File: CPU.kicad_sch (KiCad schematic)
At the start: 56 parts, among them Y1 X322524MKB4SI

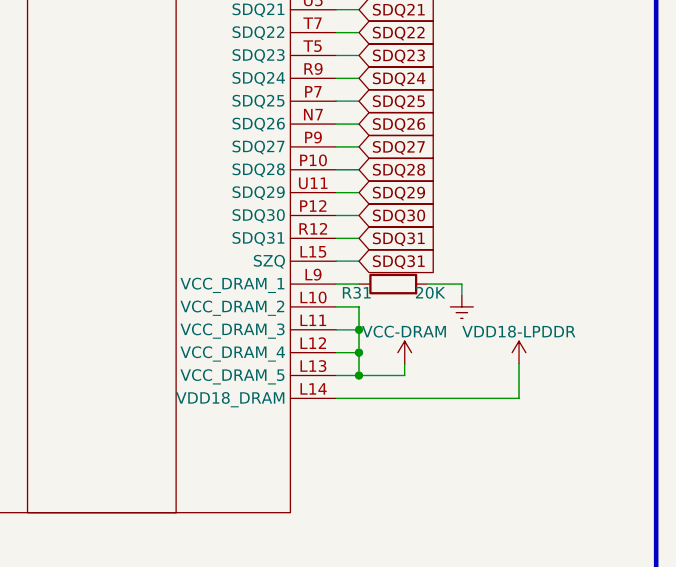
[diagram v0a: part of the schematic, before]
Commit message: Пытаюсь сделать трассировку DDК
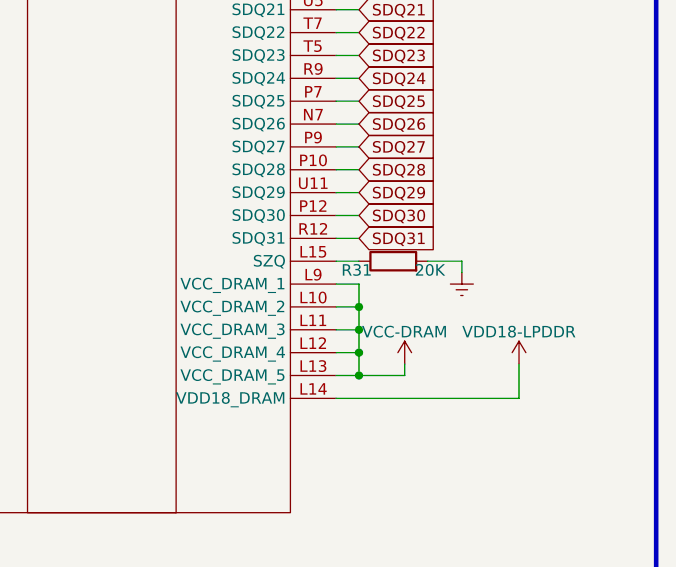
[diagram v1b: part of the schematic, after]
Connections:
- net SDQ31: no longer DD1.L15 (SZQ)
- net VCC-DRAM: now also DD1.L9 (VCC_DRAM_1)
- net at R31.1: now also DD1.L15 (SZQ); no longer DD1.L9 (VCC_DRAM_1)
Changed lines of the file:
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@@
 	)
 	(junction
+		(at 369.57 149.86)
+		(diameter 0)
+		(color 0 0 0 0)
+	)
+	(junction
 		(at 260.35 228.6)
 		(diameter 0)
@@
 	(wire
 		(pts
+			(xy 369.57 147.32) (xy 369.57 149.86)
+		)
+		(stroke
+			(width 0)
+			(type default)
+		)
+	)
+	(wire
+		(pts
 			(xy 254 228.6) (xy 260.35 228.6)
 		)
@@
 	(wire
 		(pts
+			(xy 367.03 147.32) (xy 369.57 147.32)
+		)
+		(stroke
+			(width 0)
+			(type default)
+		)
+	)
+	(wire
+		(pts
 			(xy 128.27 68.58) (xy 125.73 68.58)
 		)
@@
 	(wire
 		(pts
+			(xy 381 146.05) (xy 381 144.78)
+		)
+		(stroke
+			(width 0)
+			(type default)
+		)
+	)
+	(wire
+		(pts
 			(xy 128.27 83.82) (xy 125.73 83.82)
 		)
@@
 	(wire
 		(pts
-			(xy 381 148.59) (xy 381 147.32)
-		)
-		(stroke
-			(width 0)
-			(type default)
-		)
-	)
-	(wire
-		(pts
 			(xy 367.03 78.74) (xy 369.57 78.74)
 		)
@@
 	(wire
 		(pts
-			(xy 381 147.32) (xy 377.19 147.32)
-		)
-		(stroke
-			(width 0)
-			(type default)
-		)
-	)
-	(wire
-		(pts
 			(xy 86.36 209.55) (xy 80.01 209.55)
 		)
@@
 	(wire
 		(pts
+			(xy 381 144.78) (xy 377.19 144.78)
+		)
+		(stroke
+			(width 0)
+			(type default)
+		)
+	)
+	(wire
+		(pts
 			(xy 66.04 180.34) (xy 77.47 180.34)
 		)
@@
 	(wire
 		(pts
-			(xy 80.01 222.25) (xy 80.01 220.98)
+			(xy 367.03 144.78) (xy 369.57 144.78)
 		)
 		(stroke
@@
 	(wire
 		(pts
-			(xy 74.93 167.64) (xy 77.47 167.64)
+			(xy 80.01 222.25) (xy 80.01 220.98)
 		)
 		(stroke
@@
 	(wire
 		(pts
-			(xy 193.04 259.08) (xy 193.04 257.81)
+			(xy 74.93 167.64) (xy 77.47 167.64)
 		)
 		(stroke
@@
 	(wire
 		(pts
-			(xy 128.27 132.08) (xy 125.73 132.08)
+			(xy 193.04 259.08) (xy 193.04 257.81)
 		)
 		(stroke
@@
 	(wire
 		(pts
-			(xy 109.22 209.55) (xy 114.3 209.55)
+			(xy 128.27 132.08) (xy 125.73 132.08)
 		)
 		(stroke
@@
 	(wire
 		(pts
-			(xy 345.44 210.82) (xy 339.09 210.82)
+			(xy 109.22 209.55) (xy 114.3 209.55)
 		)
 		(stroke
@@
 	(wire
 		(pts
-			(xy 247.65 118.11) (xy 250.19 118.11)
+			(xy 345.44 210.82) (xy 339.09 210.82)
 		)
 		(stroke
@@
 	(wire
 		(pts
-			(xy 367.03 147.32) (xy 369.57 147.32)
+			(xy 247.65 118.11) (xy 250.19 118.11)
 		)
 		(stroke
@@
 	(wire
 		(pts
-			(xy 367.03 144.78) (xy 369.57 144.78)
-		)
-		(stroke
-			(width 0)
-			(type default)
-		)
-	)
-	(wire
-		(pts
 			(xy 234.95 227.33) (xy 234.95 228.6)
 		)
@@
 		)
 	)
-	(global_label "SDQ31"
-		(shape input)
-		(at 369.57 144.78 0)
-		(fields_autoplaced yes)
-		(effects
-			(font
-				(size 1.27 1.27)
-			)
-			(justify left)
-		)
-		(property "Intersheetrefs" "${INTERSHEET_REFS}"
-			(at 375.5413 144.78 0)
-			(effects
-				(font
-					(size 1.27 1.27)
-				)
-				(justify left)
-				(hide yes)
-			)
-		)
-	)
 	(global_label "SDQ30"
 		(shape input)
@@
 	)
 	(symbol
+		(lib_id "power:Earth")
+		(at 381 146.05 0)
+		(unit 1)
+		(exclude_from_sim no)
+		(in_bom yes)
+		(on_board yes)
+		(dnp no)
+		(fields_autoplaced yes)
+		(property "Reference" "#PWR0135"
+			(at 381 152.4 0)
+			(effects
+				(font
+					(size 1.27 1.27)
+				)
+				(hide yes)
+			)
+		)
+		(property "Value" "Earth"
+			(at 381 151.13 0)
+			(effects
+				(font
+					(size 1.27 1.27)
+				)
+				(hide yes)
+			)
+		)
+		(property "Footprint" ""
+			(at 381 146.05 0)
+			(effects
+				(font
+					(size 1.27 1.27)
+				)
+				(hide yes)
+			)
+		)
+		(property "Datasheet" "~"
+			(at 381 146.05 0)
+			(effects
+				(font
+					(size 1.27 1.27)
+				)
+				(hide yes)
+			)
+		)
+		(property "Description" "Power symbol creates a global label with name \"Earth\""
+			(at 381 146.05 0)
+			(effects
+				(font
+					(size 1.27 1.27)
+				)
+				(hide yes)
+			)
+		)
+		(pin "1"
+		)
+		(instances
+			(project "Sodimm-force"
+				(path "/b3673bfd-24d8-4789-b63c-c3654dc2bb6e/7bdf4494-d64d-40da-b2e3-dae4f35a6c46"
+					(reference "#PWR0135")
+					(unit 1)
+				)
+			)
+		)
+	)
+	(symbol
 		(lib_id "power:+3V8")
 		(at 339.09 201.93 0)
@@
 	(symbol
 		(lib_id "power:Earth")
-		(at 381 148.59 0)
-		(unit 1)
-		(exclude_from_sim no)
-		(in_bom yes)
-		(on_board yes)
-		(dnp no)
-		(fields_autoplaced yes)
-		(property "Reference" "#PWR0135"
-			(at 381 154.94 0)
-			(effects
-				(font
-					(size 1.27 1.27)
-				)
-				(hide yes)
-			)
-		)
-		(property "Value" "Earth"
-			(at 381 153.67 0)
-			(effects
-				(font
-					(size 1.27 1.27)
-				)
-				(hide yes)
-			)
-		)
-		(property "Footprint" ""
-			(at 381 148.59 0)
-			(effects
-				(font
-					(size 1.27 1.27)
-				)
-				(hide yes)
-			)
-		)
-		(property "Datasheet" "~"
-			(at 381 148.59 0)
-			(effects
-				(font
-					(size 1.27 1.27)
-				)
-				(hide yes)
-			)
-		)
-		(property "Description" "Power symbol creates a global label with name \"Earth\""
-			(at 381 148.59 0)
-			(effects
-				(font
-					(size 1.27 1.27)
-				)
-				(hide yes)
-			)
-		)
-		(pin "1"
-		)
-		(instances
-			(project "Sodimm-force"
-				(path "/b3673bfd-24d8-4789-b63c-c3654dc2bb6e/7bdf4494-d64d-40da-b2e3-dae4f35a6c46"
-					(reference "#PWR0135")
-					(unit 1)
-				)
-			)
-		)
-	)
-	(symbol
-		(lib_id "power:Earth")
 		(at 234.95 237.49 0)
 		(unit 1)
@@
 	)
 	(symbol
+		(lib_id "Device:R")
+		(at 373.38 144.78 90)
+		(unit 1)
+		(exclude_from_sim no)
+		(in_bom yes)
+		(on_board yes)
+		(dnp no)
+		(property "Reference" "R31"
+			(at 369.316 145.796 90)
+			(effects
+				(font
+					(size 1.27 1.27)
+				)
+			)
+		)
+		(property "Value" "20K"
+			(at 377.444 145.796 90)
+			(effects
+				(font
+					(size 1.27 1.27)
+				)
+			)
+		)
+		(property "Footprint" "Resistor_SMD:R_0402_1005Metric"
+			(at 373.38 146.558 90)
+			(effects
+				(font
+					(size 1.27 1.27)
+				)
+				(hide yes)
+			)
+		)
+		(property "Datasheet" "~"
+			(at 373.38 144.78 0)
+			(effects
+				(font
+					(size 1.27 1.27)
+				)
+				(hide yes)
+			)
+		)
+		(property "Description" "Resistor"
+			(at 373.38 144.78 0)
+			(effects
+				(font
+					(size 1.27 1.27)
+				)
+				(hide yes)
+			)
+		)
+		(pin "1"
+		)
+		(pin "2"
+		)
+		(instances
+			(project "Sodimm-force"
+				(path "/b3673bfd-24d8-4789-b63c-c3654dc2bb6e/7bdf4494-d64d-40da-b2e3-dae4f35a6c46"
+					(reference "R31")
+					(unit 1)
+				)
+			)
+		)
+	)
+	(symbol
 		(lib_id "power:+3V8")
 		(at 295.91 201.93 0)
@@
 					(unit 1)
 				)
-			)
-		)
-	)
-	(symbol
-		(lib_id "Device:R")
-		(at 373.38 147.32 90)
-		(unit 1)
-		(exclude_from_sim no)
-		(in_bom yes)
-		(on_board yes)
-		(dnp no)
-		(property "Reference" "R31"
-			(at 369.316 148.336 90)
-			(effects
-				(font
-					(size 1.27 1.27)
-				)
-			)
-		)
-		(property "Value" "20K"
-			(at 377.444 148.336 90)
-			(effects
-				(font
-					(size 1.27 1.27)
-				)
-			)
-		)
-		(property "Footprint" "Resistor_SMD:R_0402_1005Metric"
-			(at 373.38 149.098 90)
-			(effects
-				(font
-					(size 1.27 1.27)
-				)
-				(hide yes)
-			)
-		)
-		(property "Datasheet" "~"
-			(at 373.38 147.32 0)
-			(effects
-				(font
-					(size 1.27 1.27)
-				)
-				(hide yes)
-			)
-		)
-		(property "Description" "Resistor"
-			(at 373.38 147.32 0)
-			(effects
-				(font
-					(size 1.27 1.27)
-				)
-				(hide yes)
-			)
-		)
-		(pin "1"
-		)
-		(pin "2"
-		)
-		(instances
-			(project "Sodimm-force"
-				(path "/b3673bfd-24d8-4789-b63c-c3654dc2bb6e/7bdf4494-d64d-40da-b2e3-dae4f35a6c46"
-					(reference "R31")
-					(unit 1)
-				)
